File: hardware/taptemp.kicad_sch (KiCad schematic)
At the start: 23 parts, among them J1 Conn_01x06_Pin, SW1 SW_Push, SW2 SW_Push, SW3 SW_Push, SW4 SW_Push, U1 MCCOG21605D6W-BNMLWI, U2 EFM32TG110F32, U3 ST25DV64K-IE8S3, Y1 Crystal

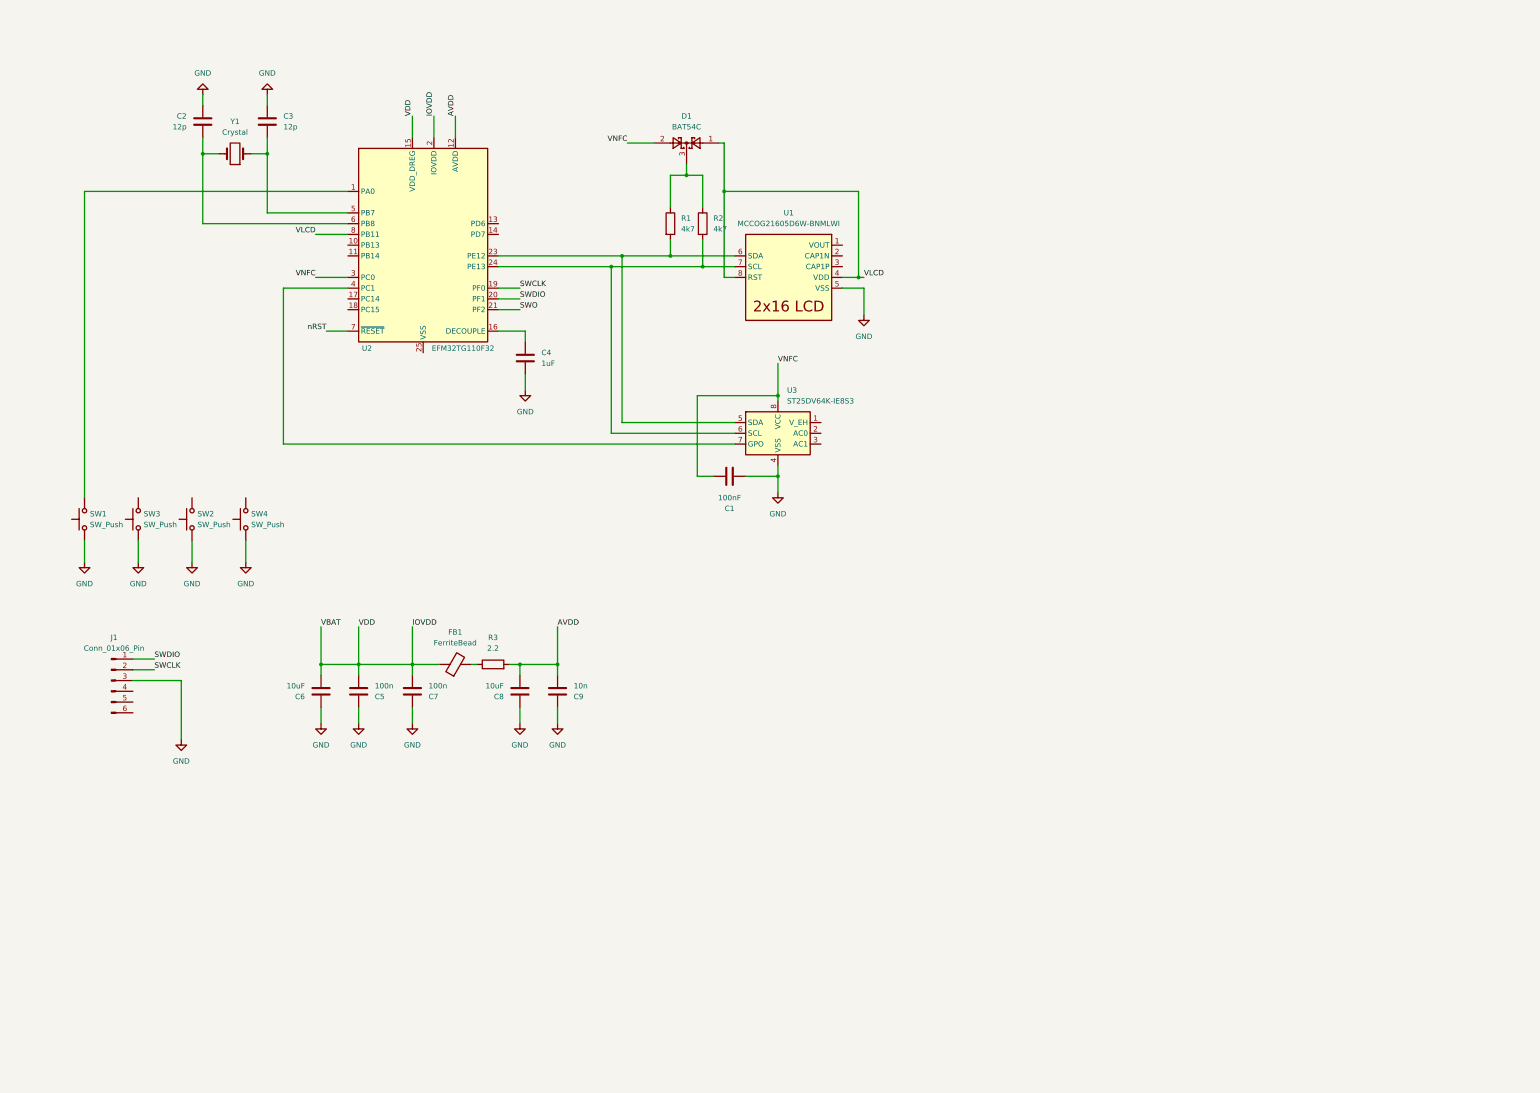
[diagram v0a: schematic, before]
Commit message: dev: initial design with stm8
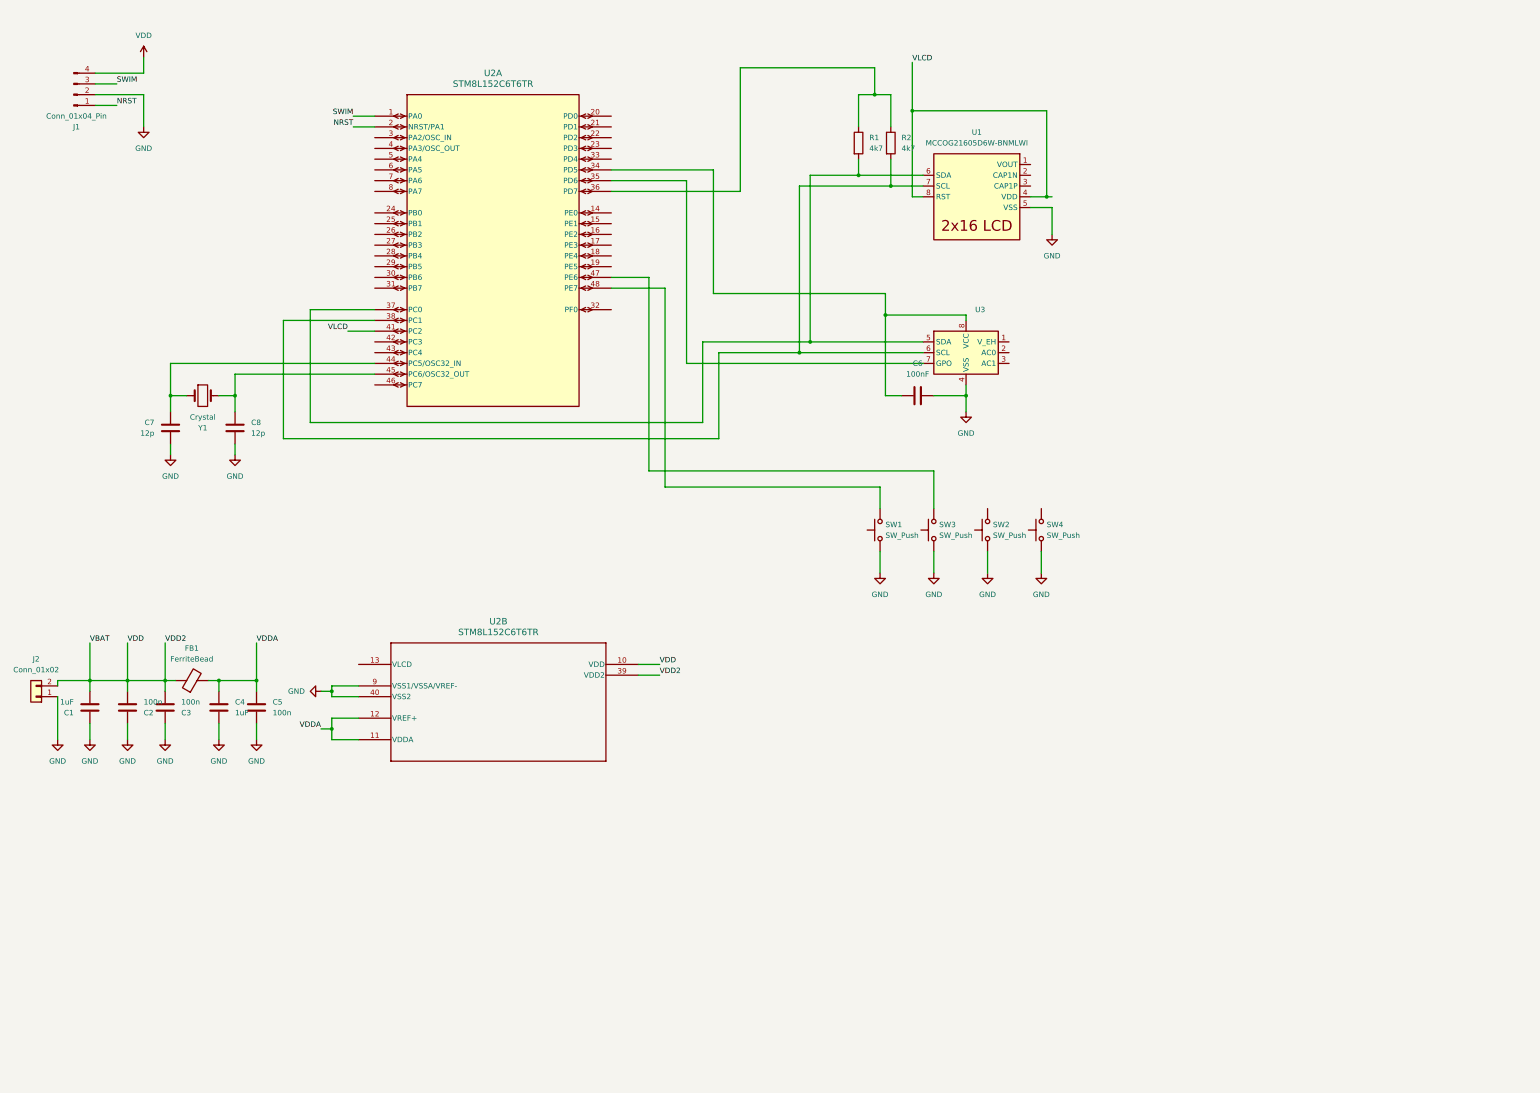
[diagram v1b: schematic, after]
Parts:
- removed C4: 1uF, Capacitor_SMD:C_0603_1608Metric_Pad1.08x0.95mm_HandSolder, symbol Device:C
- removed D1: BAT54C, Package_TO_SOT_SMD:SOT-23, symbol Diode:BAT54C
- removed J1: Conn_01x06_Pin, symbol Connector:Conn_01x06_Pin
- removed R3: 2.2, Resistor_SMD:R_0603_1608Metric_Pad0.98x0.95mm_HandSolder, symbol Device:R
- removed U2: EFM32TG110F32, Package_DFN_QFN:QFN-24-1EP_5x5mm_P0.65mm_EP3.6x3.6mm, symbol TAPTEMP:EFM32TG110F32-QFN24
- removed U3: ST25DV64K-IE8S3, Package_SO:SOIC-8_5.3x5.3mm_P1.27mm, symbol RF_NFC:ST25DV64K-IER8C3
- added J1: Conn_01x04_Pin, Connector_PinHeader_2.54mm:PinHeader_1x04_P2.54mm_Horizontal, symbol Connector:Conn_01x04_Pin
- added J2: Conn_01x02, Connector_JST:JST_PH_B2B-PH-SM4-TB_1x02-1MP_P2.00mm_Vertical, symbol Connector_Generic:Conn_01x02
- added U2: STM8L152C6T6TR, Package_QFP:LQFP-48_7x7mm_P0.5mm, symbol TAPTEMP:STM8L152C6T6TR
- added U3: ~, Package_SO:SO-8_3.9x4.9mm_P1.27mm, symbol TAPTEMP:ST25DV64KIERS
- C1: renamed from C6; value 10uF -> 1uF
- C4: renamed from C8; value 10uF -> 1uF
- C5: renamed from C9; value 10n -> 100n
- renumbered C5 to C2, C7 to C3, C1 to C6, C3 to C7, C2 to C8
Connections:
- net AVDD is gone; now on net VDDA: C4.2, C5.2
- net GND: now also J1.2 (Pin_2), J2.1 (Pin_1), U2.40 (VSS2), U2.9 (VSS1/VSSA/VREF-), U3.4 (VSS)
- net VLCD: now also U2.41 (PC2)
- net VDDA: now reaches FB1.2
- net VDDA: now also U2.11 (VDDA), U2.12 (VREF+)
- net at R1.2, U1.6 (SDA): now also U2.37 (PC0), U3.5 (SDA)
- net at R2.2, U1.7 (SCL): now also U2.38 (PC1), U3.6 (SCL)
- net at R1.1, R2.1: now also U2.36 (PD7)
- net at SW3.2: now also U2.47 (PE6)
- net at SW1.2: now also U2.48 (PE7)
- net at C7.2, Y1.1: now also U2.44 (PC5/OSC32_IN)
- net at C8.2, Y1.2: now also U2.45 (PC6/OSC32_OUT)
- net IOVDD renamed VDD
- net VDD: now also J1.4 (Pin_4), J2.2 (Pin_2), U2.10 (VDD), U2.39 (VDD2)
- net VNFC: no longer names the net of C6.2
- net VNFC: now also U2.34 (PD5), U3.8 (VCC)
- new net: U2.35 (PD6), U3.7 (GPO)
- new net NRST: J1.1 (Pin_1), U2.2 (NRST/PA1)
- new net SWIM: J1.3 (Pin_3), U2.1 (PA0)
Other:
- moved on the sheet: C1, C2, C3, C4, C5, C6, C7, C8, FB1, R1, R2, SW1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

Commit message: dev: completed routing
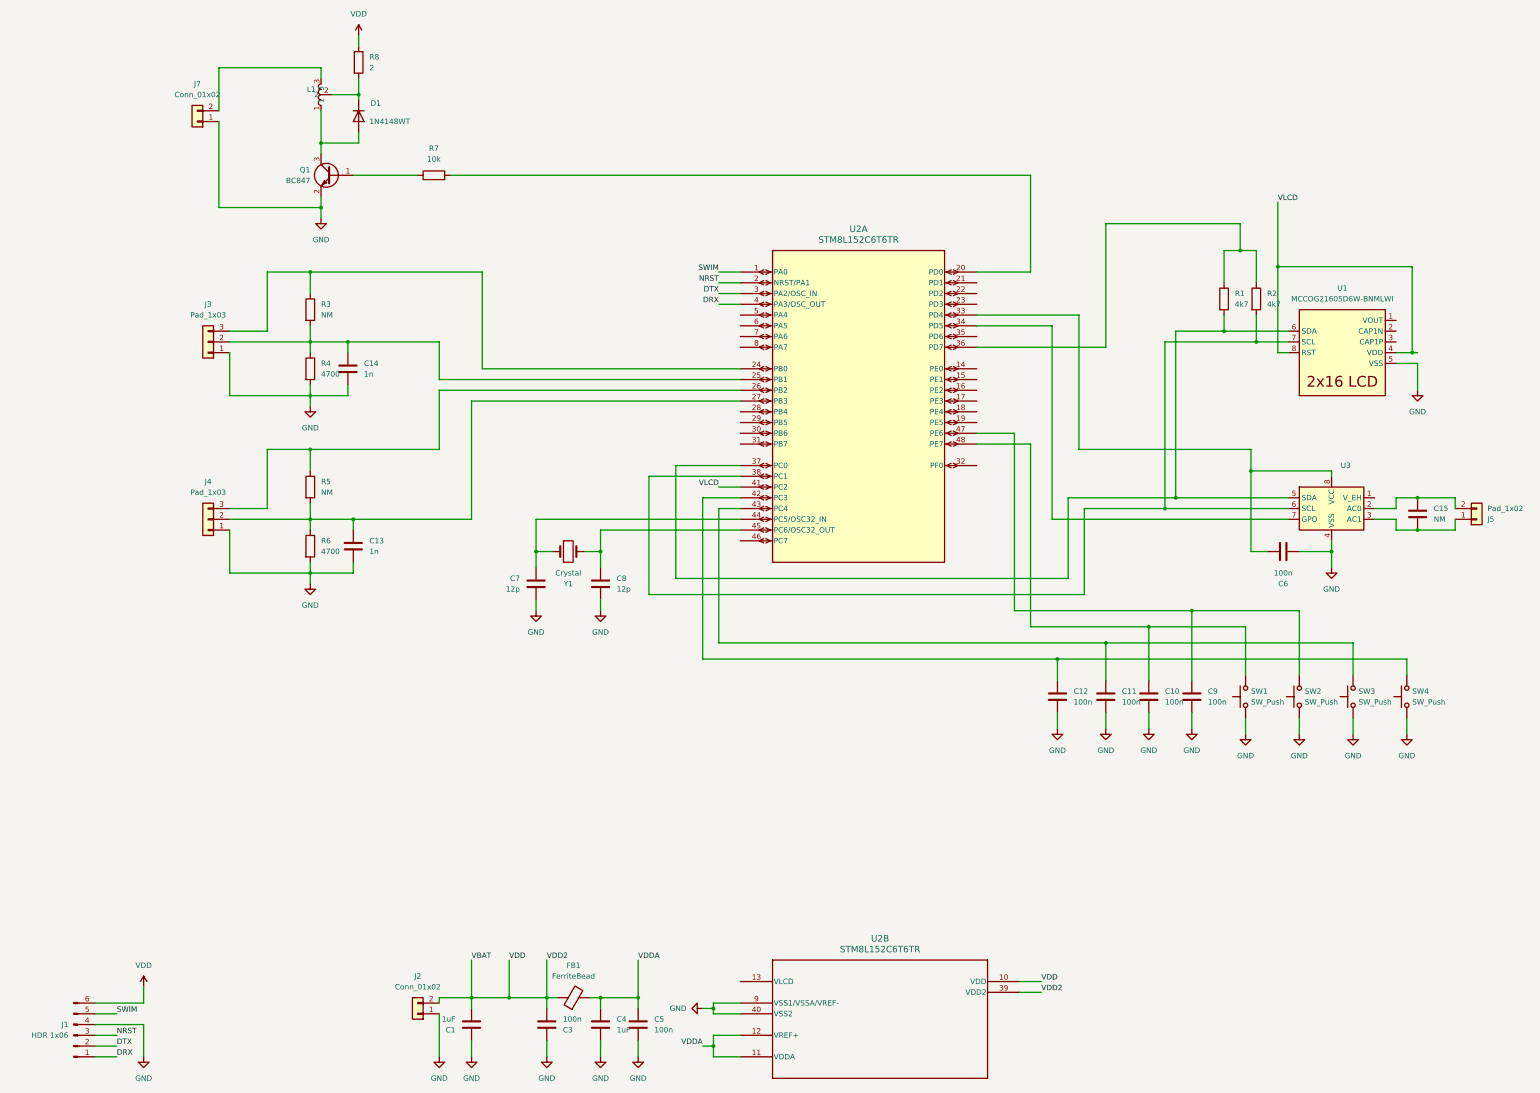
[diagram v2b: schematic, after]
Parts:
- removed C2: 100n, Capacitor_SMD:C_0603_1608Metric_Pad1.08x0.95mm_HandSolder, symbol Device:C
- added C10, C11, C12, C9: 100n, Capacitor_SMD:C_0603_1608Metric_Pad1.08x0.95mm_HandSolder, symbol Device:C
- added C13, C14: 1n, Capacitor_SMD:C_0603_1608Metric_Pad1.08x0.95mm_HandSolder, symbol Device:C
- added C15: NM, Capacitor_SMD:C_0603_1608Metric_Pad1.08x0.95mm_HandSolder, symbol Device:C
- added D1: 1N4148WT, Diode_SMD:D_SOD-523, symbol Diode:1N4148WT
- added J3, J4: Pad_1x03, TapTemp:Pad1x03, symbol Connector_Generic:Conn_01x03
- added J5: Pad_1x02, TapTemp:Pad1x02, symbol Connector_Generic:Conn_01x02
- added J7: Conn_01x02, TapTemp:Pad1x02, symbol Connector_Generic:Conn_01x02
- added L1: ~, TapTemp:Pad1x03, symbol TapTemp:L-Tapped
- added Q1: BC847, Package_TO_SOT_SMD:SOT-23, symbol Transistor_BJT:BC847
- added R3, R5: NM, Resistor_SMD:R_0603_1608Metric_Pad0.98x0.95mm_HandSolder, symbol Device:R
- added R4, R6: 4700, Resistor_SMD:R_0603_1608Metric_Pad0.98x0.95mm_HandSolder, symbol Device:R
- added R7: 10k, Resistor_SMD:R_0603_1608Metric_Pad0.98x0.95mm_HandSolder, symbol Device:R
- added R8: 2, Resistor_SMD:R_0603_1608Metric_Pad0.98x0.95mm_HandSolder, symbol Device:R
- C6: value 100nF -> 100n
- J1: value Conn_01x04_Pin -> HDR 1x06; footprint Connector_PinHeader_2.54mm:PinHeader_1x04_P2.54mm_Horizontal -> Connector_PinHeader_2.54mm:PinHeader_1x06_P2.54mm_Horizontal; symbol Connector:Conn_01x04_Pin -> Connector:Conn_01x06_Pin
- J2: footprint Connector_JST:JST_PH_B2B-PH-SM4-TB_1x02-1MP_P2.00mm_Vertical -> Connector_JST:JST_PH_S2B-PH-SM4-TB_1x02-1MP_P2.00mm_Horizontal
- U1: footprint MIDAS:MCCOG21605D6W -> TapTemp:MCCOG21605D6W
- renumbered SW3 to SW2, SW2 to SW3
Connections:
- net GND: now also J1.4 (Pin_4), C10.2, C11.2, C12.2, C13.2, C14.2, C9.2, J3.1 (Pin_1), J4.1 (Pin_1), J7.1 (Pin_1), Q1.2 (E), R4.2, R6.2; no longer J1.2 (Pin_2)
- net NRST: now also J1.3 (Pin_3); no longer J1.1 (Pin_1)
- net SWIM: now also J1.5 (Pin_5); no longer J1.3 (Pin_3)
- net VDD: now also J1.6 (Pin_6), R8.1; no longer J1.4 (Pin_4)
- net at U2.20 (PD0): now also R7.2
- net at U2.24 (PB0): now also J3.3 (Pin_3), R3.1
- net at U2.25 (PB1): now also C14.1, J3.2 (Pin_2), R3.2, R4.1
- net at U2.26 (PB2): now also J4.3 (Pin_3), R5.1
- net at U2.27 (PB3): now also C13.1, J4.2 (Pin_2), R5.2, R6.1
- net DTX: now reaches U2.3 (PA2/OSC_IN)
- net DTX: now also J1.2 (Pin_2)
- net at U2.33 (PD4): now also C6.2, U3.8 (VCC)
- net at U3.7 (GPO): now also U2.34 (PD5); no longer U2.35 (PD6)
- net DRX: now reaches U2.4 (PA3/OSC_OUT)
- net DRX: now also J1.1 (Pin_1)
- net at U2.42 (PC3): now also SW4.2, C12.1
- net at U2.43 (PC4): now also SW3.2, C11.1
- net at SW2.2, U2.47 (PE6): now also C9.1
- net at SW1.2, U2.48 (PE7): now also C10.1
- net at U3.2 (AC0): now also C15.1, J5.2 (Pin_2)
- net at U3.3 (AC1): now also C15.2, J5.1 (Pin_1)
- new net: D1.2 (A), L1.1, Q1.3 (C)
- new net: D1.1 (K), L1.2, R8.2
- new net: J7.2 (Pin_2), L1.3
- new net: Q1.1 (B), R7.1
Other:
- moved on the sheet: C1, C3, C4, C5, C6, C7, C8, FB1, J2, R1, R2, SW1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
